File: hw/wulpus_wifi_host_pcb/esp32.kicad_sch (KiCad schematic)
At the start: 3 parts, among them U4 XIAO-ESP32-C6-SMD

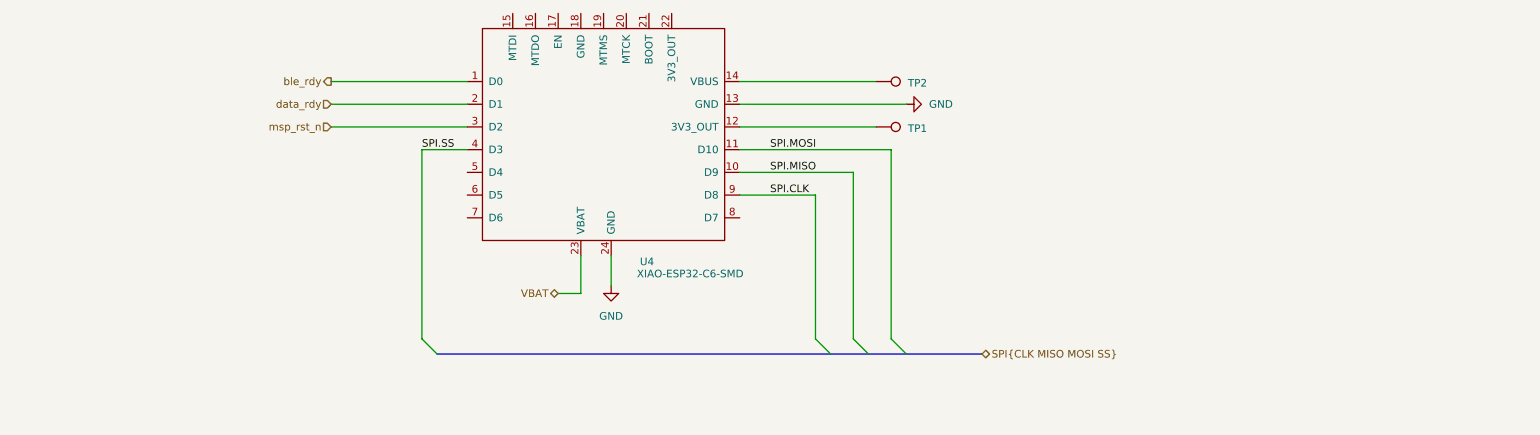
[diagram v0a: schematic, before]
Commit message: Updated footprints, mapped 3D models, added layerstack, partial placement and layout
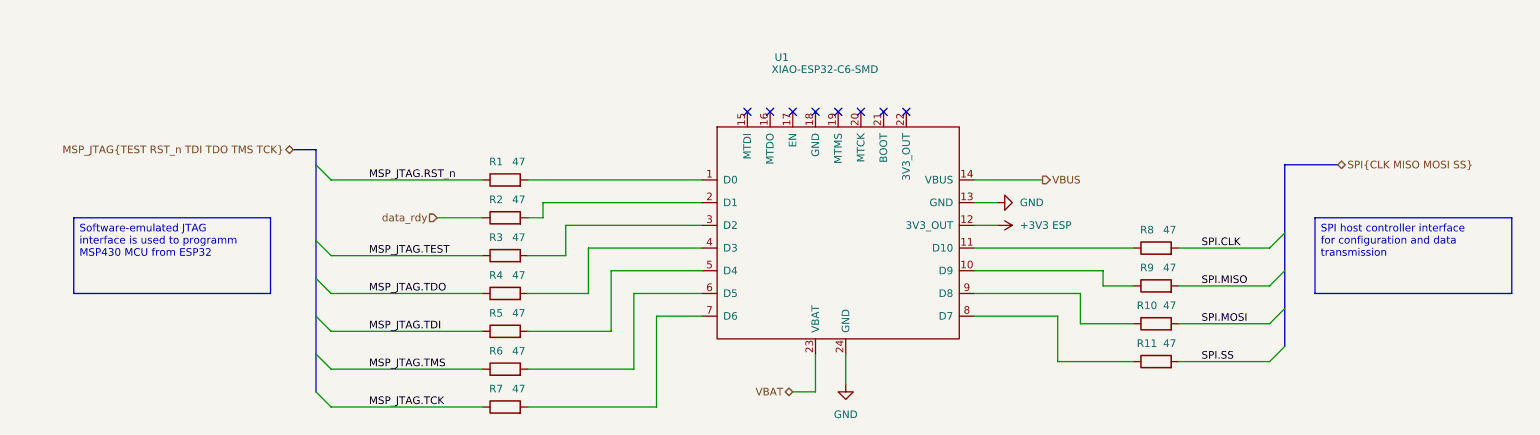
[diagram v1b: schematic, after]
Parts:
- removed TP1, TP2: TestPoint, TestPoint:TestPoint_Pad_1.5x1.5mm, symbol Connector:TestPoint
- added R1, R10, R11, R2, R3, R4, R5, R6, R7, R8, R9: 47, Resistor_SMD:R_0402_1005Metric, symbol Device:R
- renumbered U4 to U1
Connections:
- net SPI.CLK: now also R8.2; no longer U1.9 (D8)
- net SPI.MISO: now also R9.2; no longer U1.10 (D9)
- net SPI.MOSI: now also R10.2; no longer U1.11 (D10)
- net SPI.SS: now also R11.2; no longer U1.4 (D3)
- net data_rdy: now also R2.1; no longer U1.2 (D1)
- net +3V3 ESP: now reaches U1.12 (3V3_OUT)
- net VBUS: now reaches U1.14 (VBUS)
- net at U1.5 (D4): now also R5.2
- net at U1.6 (D5): now also R6.2
- net at U1.7 (D6): now also R7.2
- net at U1.8 (D7): now also R11.1
- net ble_rdy: no longer names the net of U1.1 (D0)
- net ble_rdy: now also R1.2
- net msp_rst_n: no longer names the net of U1.3 (D2)
- net msp_rst_n: now also R3.2
- new net: R8.1, U1.11 (D10)
- new net: R10.1, U1.9 (D8)
- new net: R2.2, U1.2 (D1)
- new net: R4.2, U1.4 (D3)
- new net: R9.1, U1.10 (D9)
- new net MSP_JTAG.RST_n: R1.1
- new net MSP_JTAG.TCK: R7.1
- new net MSP_JTAG.TDI: R5.1
- new net MSP_JTAG.TDO: R4.1
- new net MSP_JTAG.TEST: R3.1
- new net MSP_JTAG.TMS: R6.1
- no-connect marks 0 -> 8
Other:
- moved on the sheet: U1
